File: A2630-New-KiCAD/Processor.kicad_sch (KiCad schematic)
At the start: 50 parts, among them U200 MC68030FE, U201 MC68882, U204 74HCT04, X1 25MHz, X2 25MHz

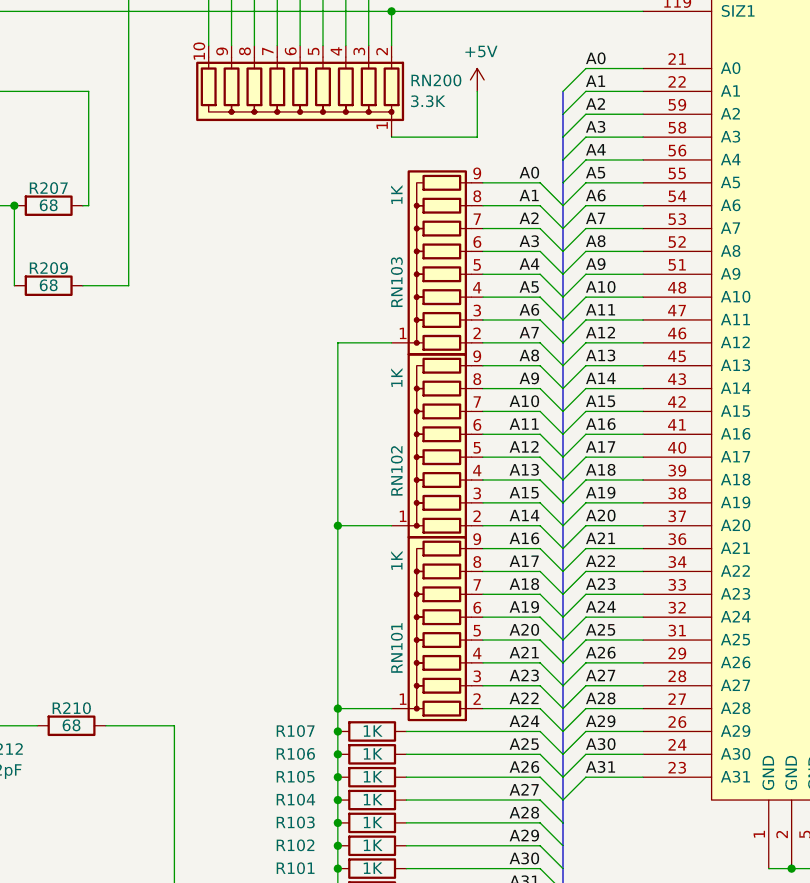
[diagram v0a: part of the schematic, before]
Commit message: Add files via upload
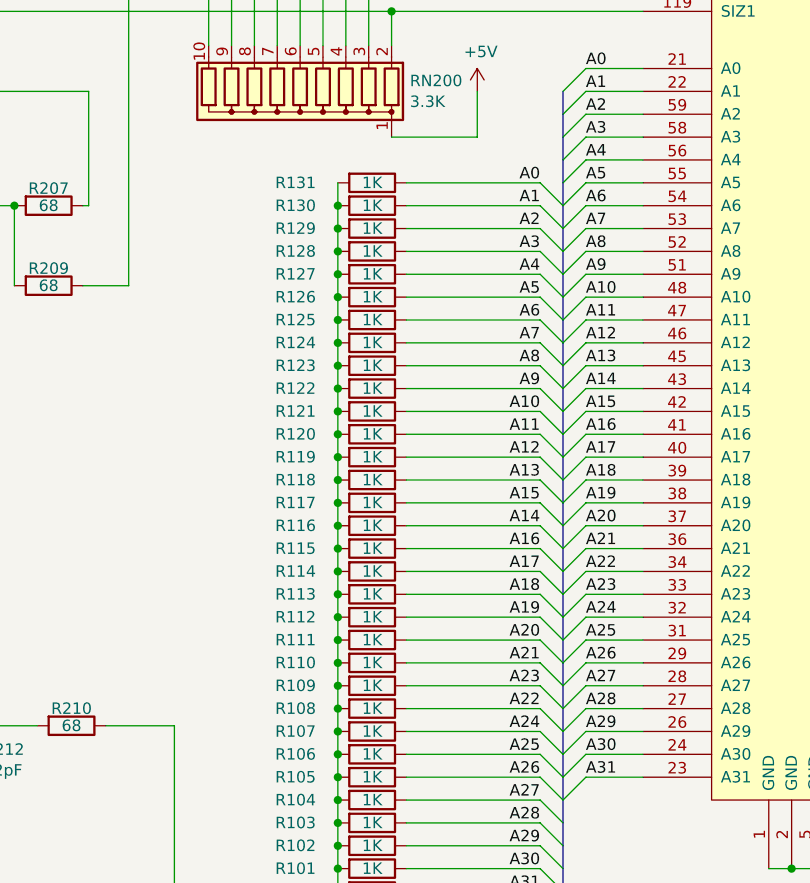
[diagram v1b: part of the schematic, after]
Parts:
- removed RN101, RN102, RN103: 1K, Resistor_THT:R_Array_SIP9, symbol Device:R_Network08
- added R108, R109, R110, R111, R112, R113, R114, R115, R116, R117, R118, R119, R120, R121, R122, R123, R124, R125, R126, R127, R128, R129, R130, R131: 1K, Resistor_SMD:R_0805_2012Metric, symbol Device:R
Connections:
- net A0: now also R131.1
- net A1: now also R130.1
- net A10: now also R121.1
- net A11: now also R120.1
- net A12: now also R119.1
- net A13: now also R118.1
- net A14: now also R116.1
- net A15: now also R117.1
- net A16: now also R115.1
- net A17: now also R114.1
- net A18: now also R113.1
- net A19: now also R112.1
- net A2: now also R129.1
- net A20: now also R111.1
- net A21: now also R110.1
- net A22: now also R108.1
- net A23: now also R109.1
- net A3: now also R128.1
- net A4: now also R127.1
- net A5: now also R126.1
- net A6: now also R125.1
- net A7: now also R124.1
- net A8: now also R123.1
- net A9: now also R122.1
- net GND: now also R108.2, R109.2, R110.2, R111.2, R112.2, R113.2, R114.2, R115.2, R116.2, R117.2, R118.2, R119.2, R120.2, R121.2, R122.2, R123.2, R124.2, R125.2, R126.2, R127.2, R128.2, R129.2, R130.2, R131.2
